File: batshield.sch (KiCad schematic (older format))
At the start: 68 parts, among them J1 Audio-Jack-2, J10 left down pins, J11 service power, J2 Audio-Jack-2, J3 mic in, J4 Audio-Jack-2, J5 DIN-5_180degree, J6 DIN-5_180degree, J7 rigth up pins, J8 left uppins, J9 rigth donw pins, SW1 SW_SPDT, SW10 SW_Push, SW11 SW_SPST, SW2 SW_SPDT, SW3 SW_SPST, SW4 SW_SPST, SW5 SW_SPST, SW6 SW_SPST, SW7 SW_Push, SW8 SW_Push, SW9 SW_Push, U1 TL072, U2 4N35

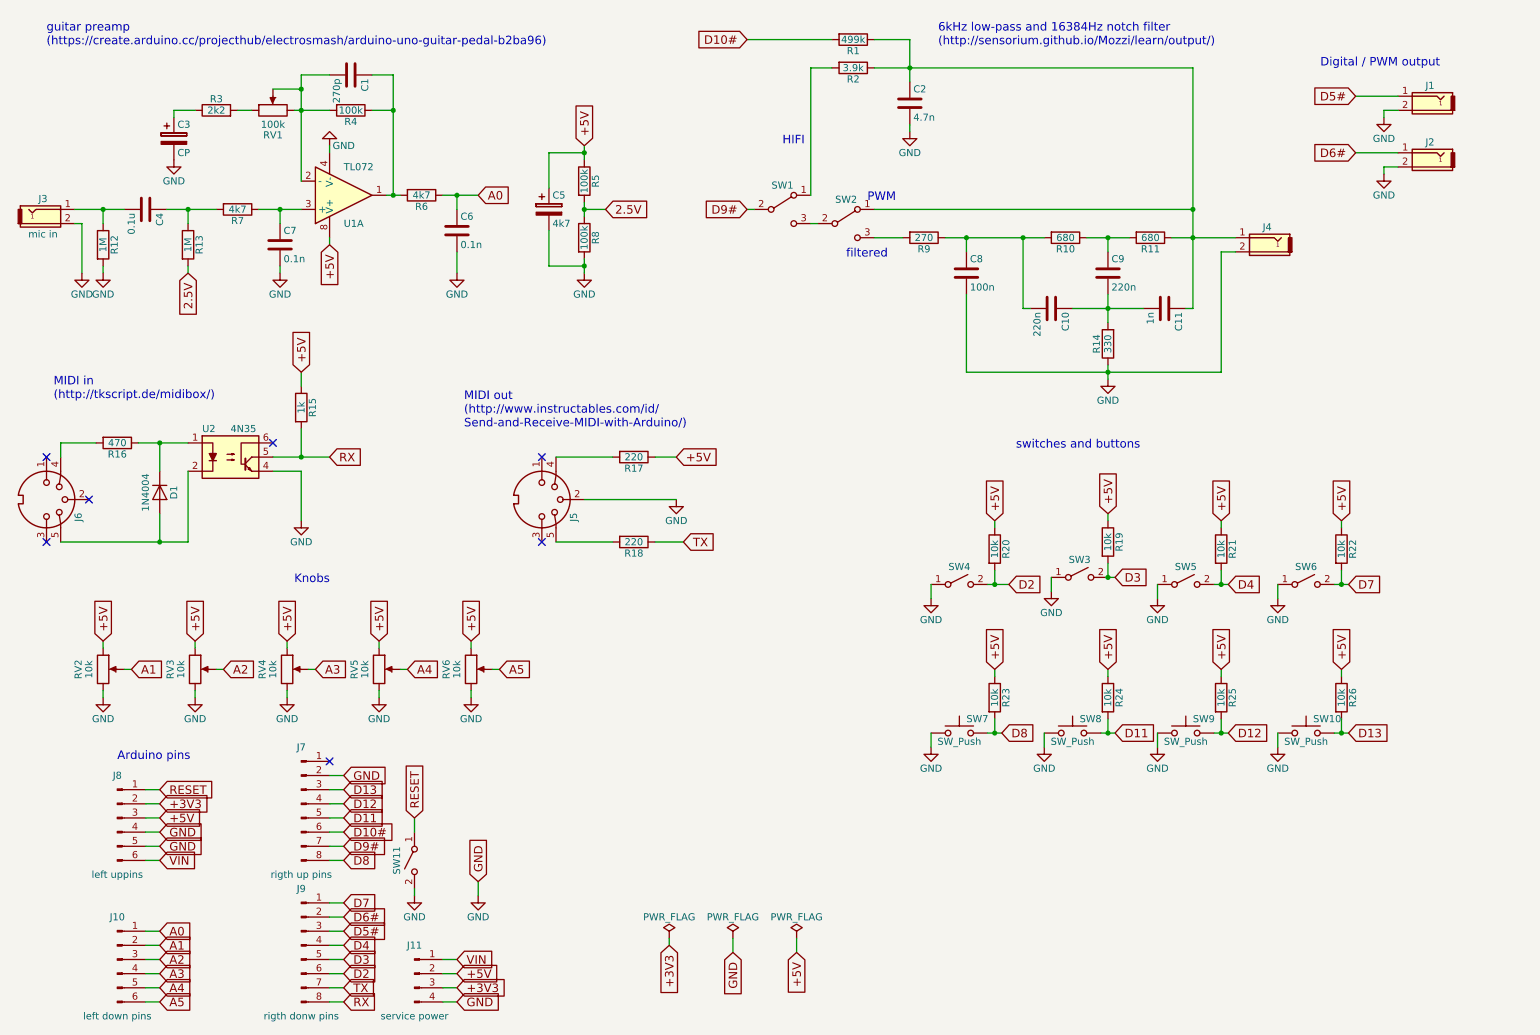
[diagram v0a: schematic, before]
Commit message: mejoras, mejoras, mejoras
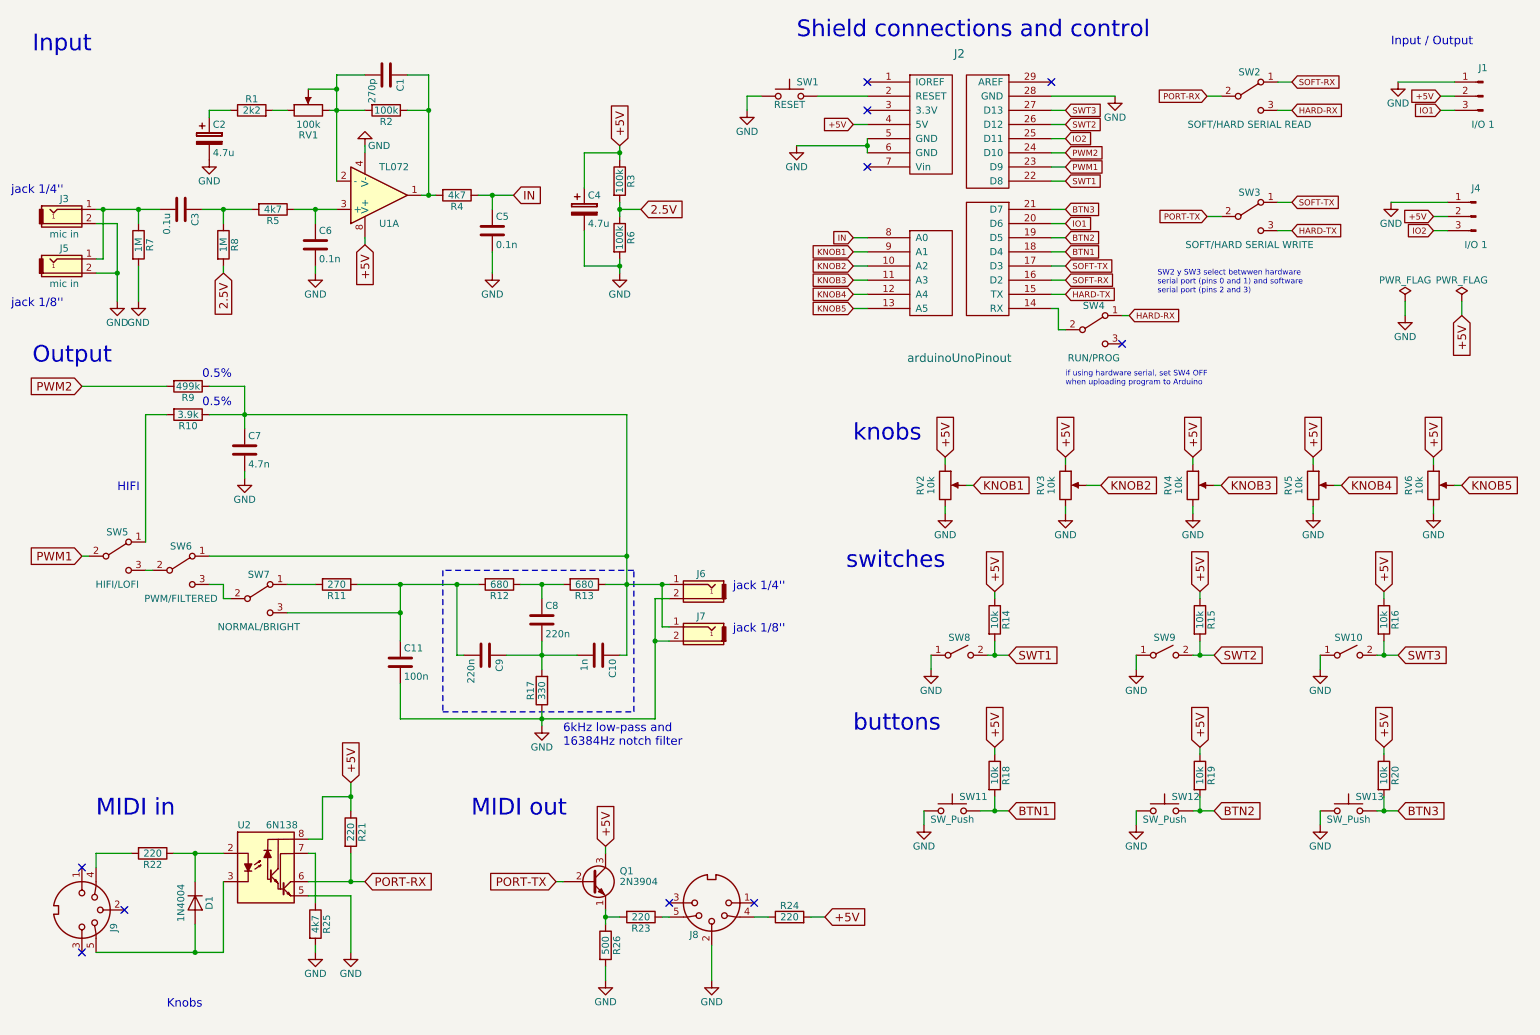
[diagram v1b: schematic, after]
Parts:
- removed J1, J2: Audio-Jack-2, symbol Audio-Jack-2
- removed J10: left down pins, symbol Conn_01x06_Male
- removed J11: service power, symbol Conn_01x04_Male
- removed J7: rigth up pins, symbol Conn_01x08_Male
- removed J8: left uppins, symbol Conn_01x06_Male
- removed J9: rigth donw pins, symbol Conn_01x08_Male
- removed R15: 1k, symbol R
- removed R22: 10k, symbol R
- removed SW10: SW_Push, symbol SW_Push
- removed SW11, SW6: SW_SPST, symbol SW_SPST
- removed U2: 4N35, Housings_DIP:DIP-6_W7.62mm, symbol 4N25
- added J1, J4: I/O 1, symbol Conn_01x03_Male
- added J2: arduinoUnoPinout, symbol arduinoUnoPinout
- added J5: mic in, symbol Audio-Jack-2
- added J7: Audio-Jack-2, symbol Audio-Jack-2
- added Q1: 2N3904, TO_SOT_Packages_THT:TO-92_Molded_Narrow, symbol 2N3904
- added R21: 220, symbol R
- added R25: 4k7, symbol R
- added SW1: RESET, symbol SW_Push
- added SW2: SOFT/HARD SERIAL READ, symbol SW_SPDT
- added SW3: SOFT/HARD SERIAL WRITE, symbol SW_SPDT
- added SW4: RUN/PROG, symbol SW_SPDT
- added SW7: NORMAL/BRIGHT, symbol SW_SPDT
- added U2: 6N138, Housings_DIP:DIP-8_W7.62mm, symbol 6N138
- C1: footprint (none) -> Capacitors_THT:C_Disc_D5.0mm_W2.5mm_P5.00mm
- C2: renamed from C3; value CP -> 4.7u
- C3: renamed from C4; footprint (none) -> Capacitors_THT:C_Disc_D5.0mm_W2.5mm_P2.50mm
- C4: renamed from C5; value 4k7 -> 4.7u
- C7: renamed from C2; footprint (none) -> Capacitors_THT:C_Disc_D5.0mm_W2.5mm_P5.00mm
- R22: renamed from R16; value 470 -> 220
- R26: value 10k -> 500
- SW5: renamed from SW1; value SW_SPDT -> HIFI/LOFI
- SW6: renamed from SW2; value SW_SPDT -> PWM/FILTERED
- renumbered C11 to C10, C8 to C11, C6 to C5, C7 to C6, C9 to C8, C10 to C9, J4 to J6, J5 to J8, J6 to J9, R3 to R1, R2 to R10, R9 to R11, R10 to R12, R11 to R13, R20 to R14, R19 to R15, R21 to R16, R14 to R17, R23 to R18, R24 to R19, R4 to R2, R25 to R20, R18 to R23, R17 to R24, R5 to R3, R6 to R4, R7 to R5, R8 to R6, R12 to R7, R13 to R8, R1 to R9, SW5 to SW10, SW7 to SW11, SW8 to SW12, SW9 to SW13, SW4 to SW8, SW3 to SW9
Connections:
- net D13 is gone; now on net GND: R26.2
- net TX is gone; now on an unnamed net: R23.1
- net +5V: now also R24.2, J1.2 (Pin_2), J2.4 (5V), J4.2 (Pin_2), Q1.3 (C), R21.1, U2.8; no longer R24.1, R26.1
- net GND: now also J1.1 (Pin_1), J2.28 (GND), J2.5 (GND), J2.6 (GND), J4.1 (Pin_1), J5.2, J7.2, R25.2, SW1.1, U2.5
- net at C11.1, C9.2, R11.1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: now also SW7.3 (C)
- net at R11.2: now also SW7.1 (A); no longer SW6.3 (C)
- net at C10.1, C7.1, J6.1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: now also J7.1
- net at D1.1 (K), R22.1: now also U2.2
- net at D1.2 (A), J9.5: now also U2.3
- net at J8.4: now also R24.1; no longer R24.2
- net at J8.5: no longer R23.2
- net at C3.2, J3.1, R7.1: now also J5.1
- net A0 renamed IN
- net IN: now also J2.8 (A0)
- net A1 renamed KNOB1
- net KNOB1: now also J2.9 (A1)
- net A2 renamed KNOB2
- net KNOB2: now also J2.10 (A2)
- net A3 renamed KNOB3
- net KNOB3: now also J2.11 (A3)
- net A4 renamed KNOB4
- net KNOB4: now also J2.12 (A4)
- net A5 renamed KNOB5
- net KNOB5: now also J2.13 (A5)
- net D10# renamed PWM2
- net PWM2: now also J2.24 (D10)
- net D11 renamed BTN2
- net BTN2: now also J2.19 (D5)
- net D12 renamed BTN3
- net BTN3: now also J2.21 (D7)
- net D2 renamed SWT1
- net SWT1: now also J2.22 (D8)
- net D3 renamed SWT2
- net SWT2: now also J2.26 (D12)
- net D4 renamed SWT3
- net SWT3: now also J2.27 (D13)
- net D8 renamed BTN1
- net BTN1: now also J2.18 (D4)
- net D9# renamed PWM1
- net PWM1: now also J2.23 (D9)
- new net: SW6.3 (C), SW7.2 (B)
- new net: Q1.1 (E), R23.2, R26.1
- new net: R25.1, U2.7
- new net: J2.14 (RX), SW4.2 (B)
- new net: J2.2 (RESET), SW1.2
- new net HARD-RX: SW2.3 (C), SW4.1 (A)
- new net HARD-TX: J2.15 (TX), SW3.3 (C)
- new net IO1: J1.3 (Pin_3), J2.20 (D6)
- new net IO2: J2.25 (D11), J4.3 (Pin_3)
- new net PORT-RX: R21.2, SW2.2 (B), U2.6
- new net PORT-TX: Q1.2 (B), SW3.2 (B)
- new net SOFT-RX: J2.16 (D2), SW2.1 (A)
- new net SOFT-TX: J2.17 (D3), SW3.1 (A)
- no-connect marks 7 -> 10
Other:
- note added: "0.5%"
- note added: "6kHz low-pass and\n16384Hz notch filter"
- note added: "Input"
- note added: "Input / Output"
- note added: "MIDI in"
- note added: "MIDI out"
- note added: "Output"
- note added: "SW2 y SW3 select betwwen hardware\nserial port (pins 0 and 1) and software\nserial port (pins 2 and 3)"
- note added: "Shield connections and control"
- note added: "buttons"
- note added: "if using hardware serial, set SW4 OFF \nwhen uploading program to Arduino"
- note added: "jack 1/4''"
- note added: "jack 1/8''"
- note added: "knobs"
- note added: "switches"
- note removed: "6kHz low-pass and 16384Hz notch filter\n(http://sensorium.github.io/Mozzi/learn/output/)"
- note removed: "Arduino pins"
- note removed: "Digital / PWM output"
- note removed: "MIDI in\n(http://tkscript.de/midibox/)"
- note removed: "MIDI out\n(http://www.instructables.com/id/\nSend-and-Receive-MIDI-with-Arduino/)"
- note removed: "PWM\n"
- note removed: "filtered"
- note removed: "guitar preamp\n(https://create.arduino.cc/projecthub/electrosmash/arduino-uno-guitar-pedal-b2ba96)"
- note removed: "switches and buttons"
- moved on the sheet: C1, C10, C11, C2, C3, C4, C5, C6, C7, C8, C9, D1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
